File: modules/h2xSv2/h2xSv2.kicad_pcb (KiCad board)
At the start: 2 copper layers, 95.2 x 40.6 mm, 19 parts, among them J1 Conn_01x10_Male, J10 Conn_01x02_Male, J11 Conn_01x06_Male, J2 Conn_01x10_Male, J3 Conn_01x10_Male, J4 Conn_01x10_Male, J5 Conn_01x04_Male, J6 Conn_01x04_Male, J7 Conn_01x12_Male, J8 Conn_01x12_Male, J9 Conn_01x12_Male

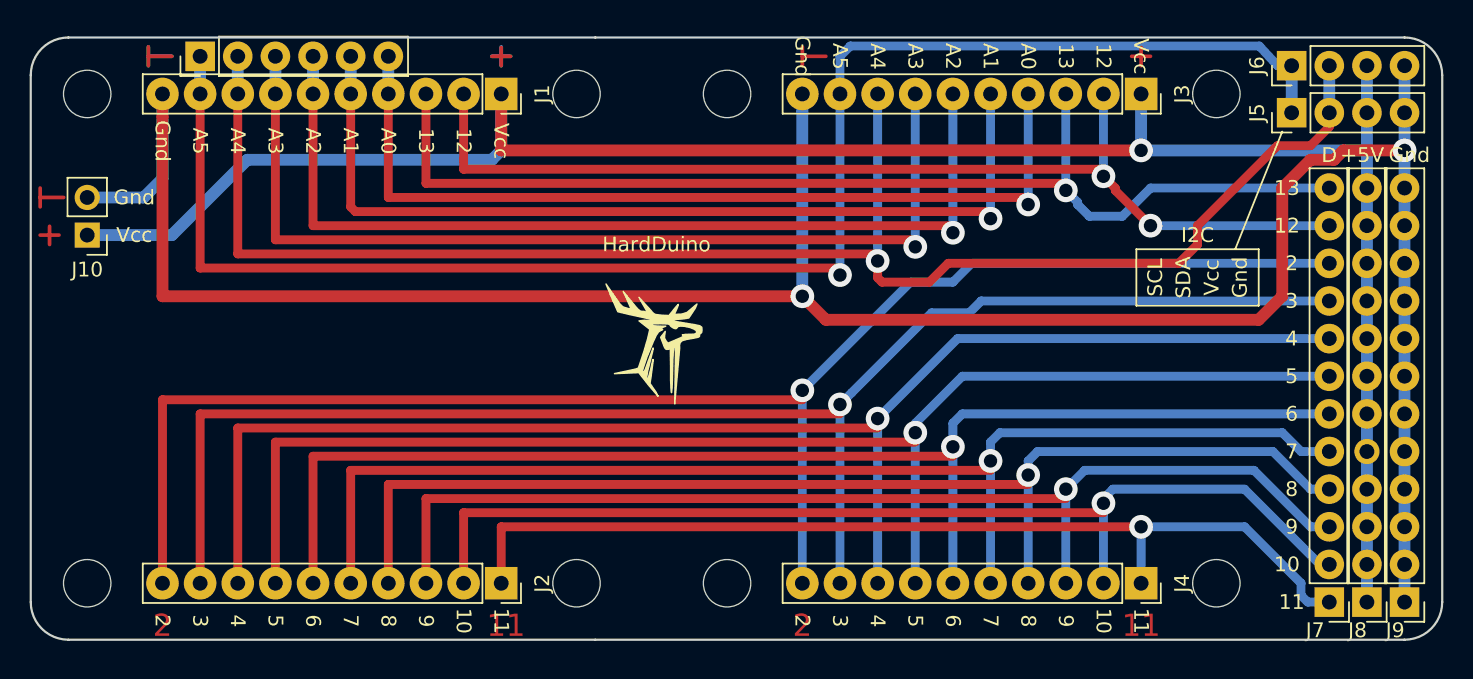
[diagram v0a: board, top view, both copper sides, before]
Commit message: Fix sizes
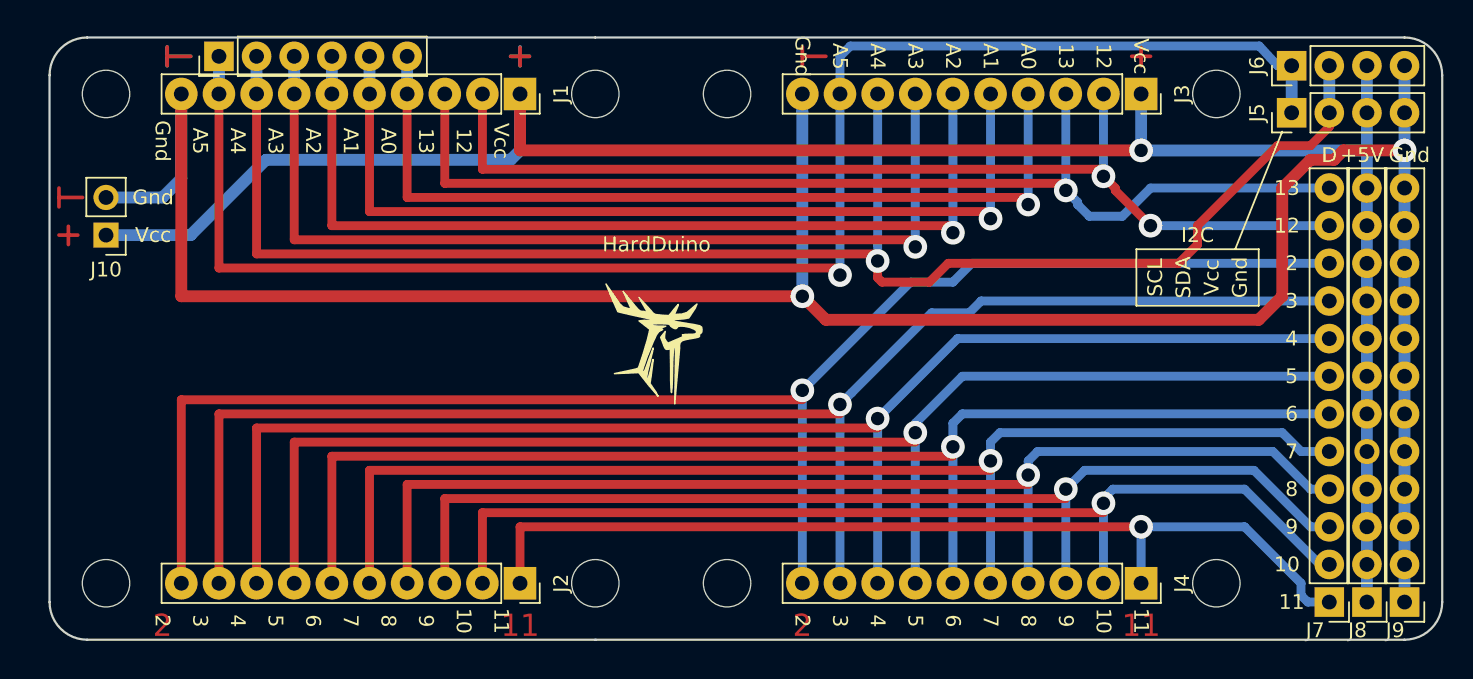
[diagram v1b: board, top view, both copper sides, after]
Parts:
- moved J11 1.27 mm to (66.0, 22.9)
- moved H1 1.27 mm to (58.4, 58.4)
- moved H3 1.27 mm to (58.4, 25.4)
- moved J10 1.27 mm to (58.4, 34.9)
- moved H2 1.27 mm to (91.4, 58.4)
- moved H4 1.27 mm to (91.4, 25.4)
- moved J1 1.27 mm to (86.4, 25.4)
- moved J2 1.27 mm to (86.4, 58.4)
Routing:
- net VCC: track 136.5 -> 135.2 mm
- net GND: track 168.3 -> 167.0 mm
- net /A5: track 106.8 -> 105.5 mm
- net /A4: track 108.7 -> 107.5 mm
- net /A3: track 65.9 -> 64.6 mm
- net /5: track 92.8 -> 91.5 mm
- net /3: track 102.6 -> 101.3 mm
- net /13: track 75.1 -> 73.8 mm
- net /12: track 70.5 -> 69.3 mm
- net /11: track 66.1 -> 64.8 mm
- net /A2: track 64.0 -> 62.7 mm
- net /A0: track 60.2 -> 58.9 mm
- net /9: track 75.1 -> 73.9 mm
- net /8: track 79.7 -> 78.5 mm
- net /7: track 84.0 -> 82.7 mm
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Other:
- board size 95.2 x 40.6 mm -> 94 x 40.6 mm
